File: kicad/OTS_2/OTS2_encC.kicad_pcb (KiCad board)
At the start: 2 copper layers, 38.1 x 38.1 mm, 20 parts

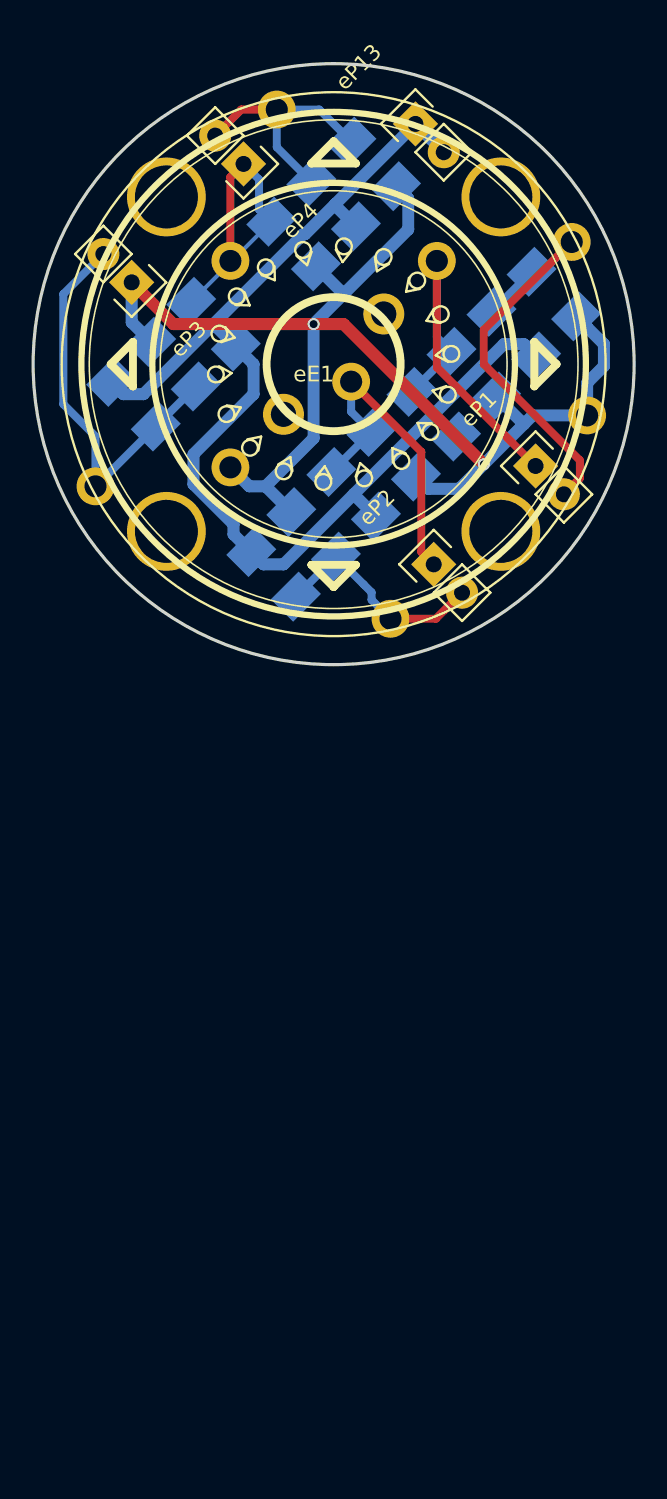
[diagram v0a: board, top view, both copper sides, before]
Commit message: gerbers for encA, encB, encC, main - ready
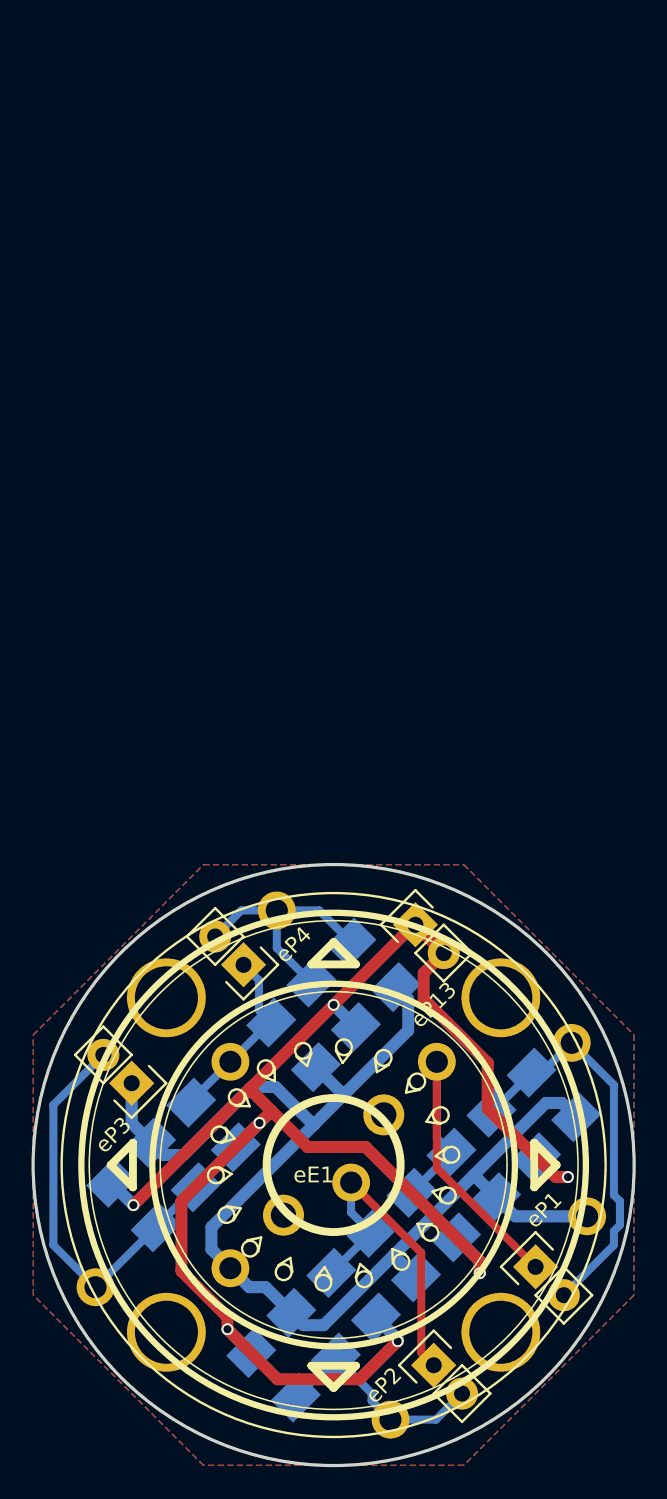
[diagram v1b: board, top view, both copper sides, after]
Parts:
- moved eC2 50.8 mm to (89.5, 120.7)
- moved eC3 50.8 mm to (95.9, 134.0)
- moved eC6 50.8 mm to (81.9, 128.3)
- moved eE1 50.8 mm to (92.1, 128.3)
- moved eR4 50.8 mm to (93.3, 136.5)
- moved eP13 50.8 mm to (97.3, 113.0)
- moved eC1 50.8 mm to (101.0, 128.9)
- moved eC4 50.8 mm to (106.0, 123.8)
- moved eC5 50.8 mm to (94.6, 115.6)
- moved eC7 50.8 mm to (90.8, 139.1)
- moved eP1 50.8 mm to (104.9, 134.7)
- moved eP2 50.8 mm to (98.4, 141.0)
- moved eP3 50.8 mm to (79.3, 123.1)
- moved eP4 50.8 mm to (86.4, 115.6)
- moved eR2 50.8 mm to (98.4, 131.4)
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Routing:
- net /eVCC: track 78.3 -> 113.0 mm, vias 0 -> 7
- net /eECB: track 18.1 -> 11.9 mm
- net /eS2: track 28.2 -> 25.7 mm
- net /eGND: track 86.1 -> 83.9 mm, vias 2 -> 0
- net /eS4: track 25.6 -> 26.1 mm
- added copper zone on B.Cu, net /eGND
- added copper zone on F.Cu, net /eVCC
